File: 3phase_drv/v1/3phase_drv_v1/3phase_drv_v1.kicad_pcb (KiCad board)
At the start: 2 copper layers, 178 x 93 mm, 40 parts, among them J1 Logic IN, J2 Supply, J3 VSenses, J4 Phases, Q1 IRF3710, Q2 IRF3710, Q3 IRF3710, Q4 IRF3710, Q5 IRF3710, Q6 IRF3710, U1 IRS2110S, U2 IRS2110S, U3 IRS2110S

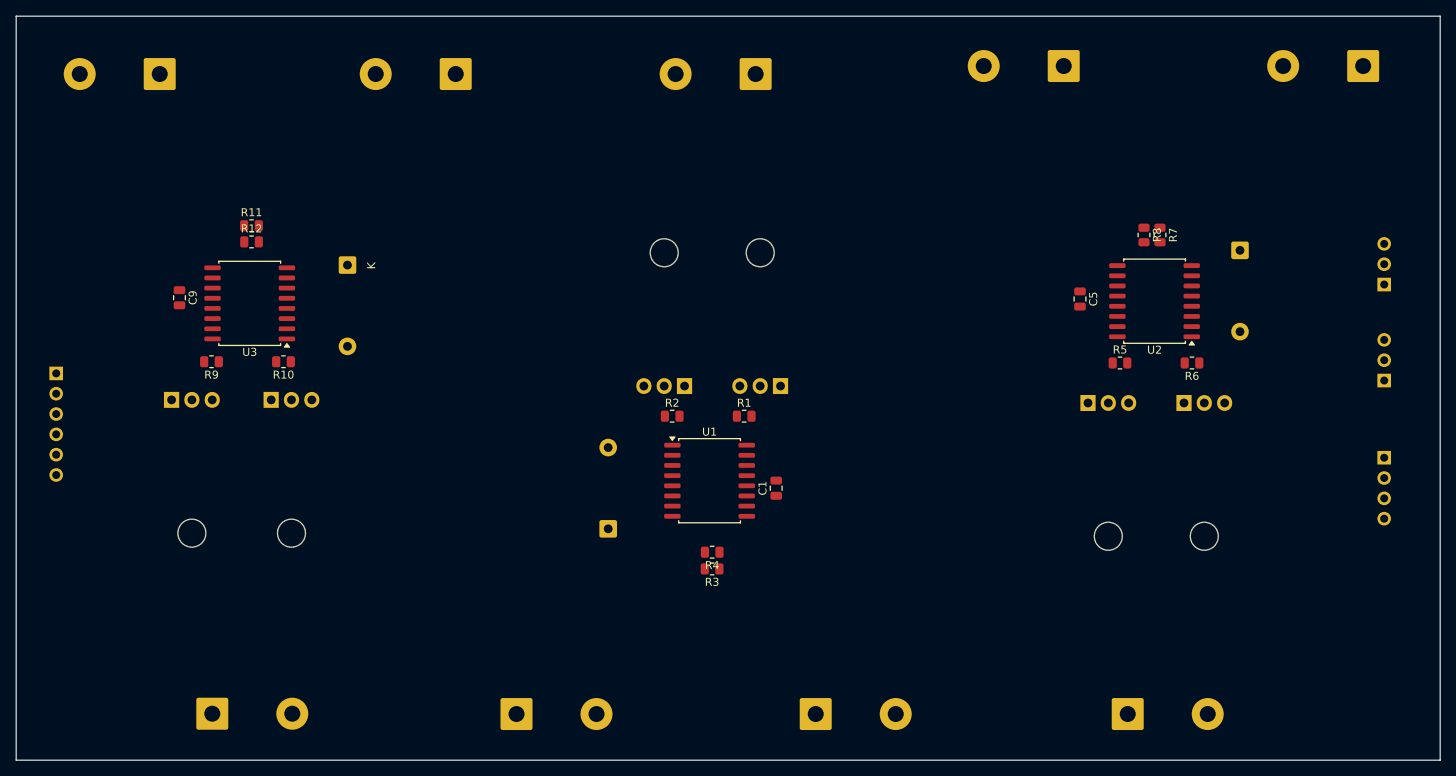
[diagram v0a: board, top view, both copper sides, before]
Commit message: re-layout and finish routing
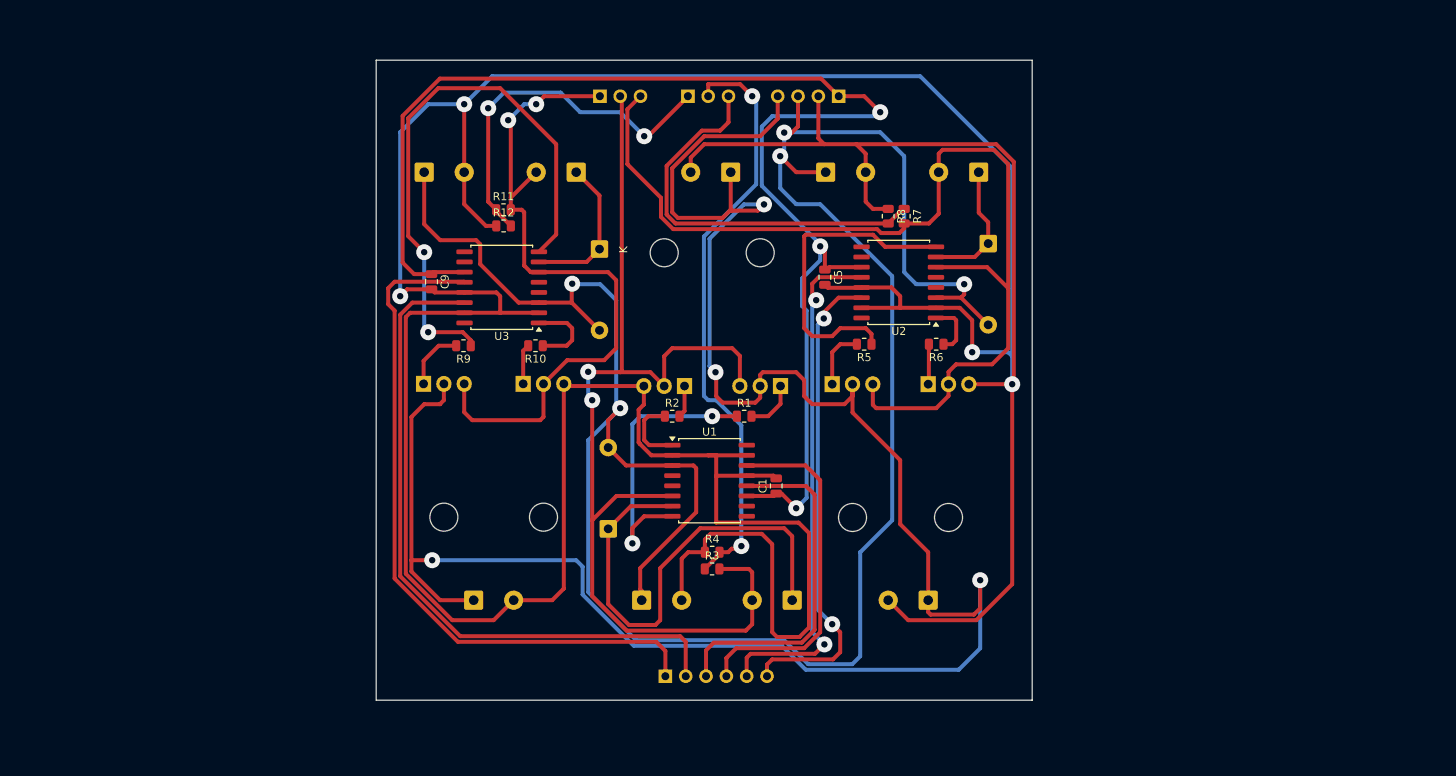
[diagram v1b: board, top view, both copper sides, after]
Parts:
- C10, C11, C12, C2, C3, C4, C6, C7, C8: footprint Capacitor_THT:CP_Radial_D35.0mm_P10.00mm_SnapIn -> Capacitor_THT:CP_Radial_D13.0mm_P5.00mm
- moved J4 100.8 mm to (140.0, 58.0), turned to -90 degrees
- moved J3 94.0 mm to (151.0, 58.0), turned to -90 degrees
- moved J1 85.0 mm to (148.2, 130.5), turned to -90 degrees
- moved J2 81.8 mm to (169.8, 58.0), turned to 90 degrees
- moved C10 53.5 mm to (137.0, 67.5)
- moved C6 49.9 mm to (187.3, 67.5)
- moved C12 35.6 mm to (124.2, 121.0)
- moved C7 32.6 mm to (168.2, 67.5), turned to 0 degrees
- moved Q3 32.1 mm to (169.0, 94.0)
- moved Q4 32.1 mm to (181.0, 94.0)
- moved R5 32.1 mm to (173.0, 89.0), turned to 180 degrees
- moved R6 32.1 mm to (182.0, 89.0)
- moved R7 32.1 mm to (178.0, 73.0)
- moved R8 32.1 mm to (176.0, 73.0)
- moved U2 32.1 mm to (177.3, 81.3)
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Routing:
- net GND: track 0.00 -> 544.0 mm, vias 0 -> 4
- net min+10V: track 0.00 -> 293.6 mm, vias 0 -> 5
- net VM: track 0.00 -> 261.2 mm, vias 0 -> 4
- net +3.3V: track 0.00 -> 173.1 mm, vias 0 -> 3
- net /IRS2110S1/Out: track 0.00 -> 135.1 mm, vias 0 -> 2
- net /IRS2110S2/Out: track 0.00 -> 129.2 mm
- net /IRS2110S/HIN: track 0.00 -> 87.3 mm
- net /IRS2110S/Out: track 0.00 -> 86.9 mm, vias 0 -> 2
- net /IRS2110S/LIN: track 0.00 -> 84.7 mm
- net /IRS2110S1/VSense: track 0.00 -> 75.2 mm, vias 0 -> 2
- net Net-(U3-HO): track 0.00 -> 71.5 mm, vias 0 -> 2
- net /IRS2110S2/HIN: track 0.00 -> 65.4 mm, vias 0 -> 2
- net /IRS2110S2/LIN: track 0.00 -> 60.7 mm, vias 0 -> 2
- net Net-(D1-K): track 0.00 -> 59.9 mm
- net /IRS2110S2/VSense: track 0.00 -> 50.3 mm
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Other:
- board size 178 x 93 mm -> 82 x 80 mm
